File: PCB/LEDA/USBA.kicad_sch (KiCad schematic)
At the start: 22 parts, among them J1 USB_A, J2 Conn_01x03, T1 T3902_MEMS_Mic, U2 ESP32-S3-MINI-1, U5 MD8942

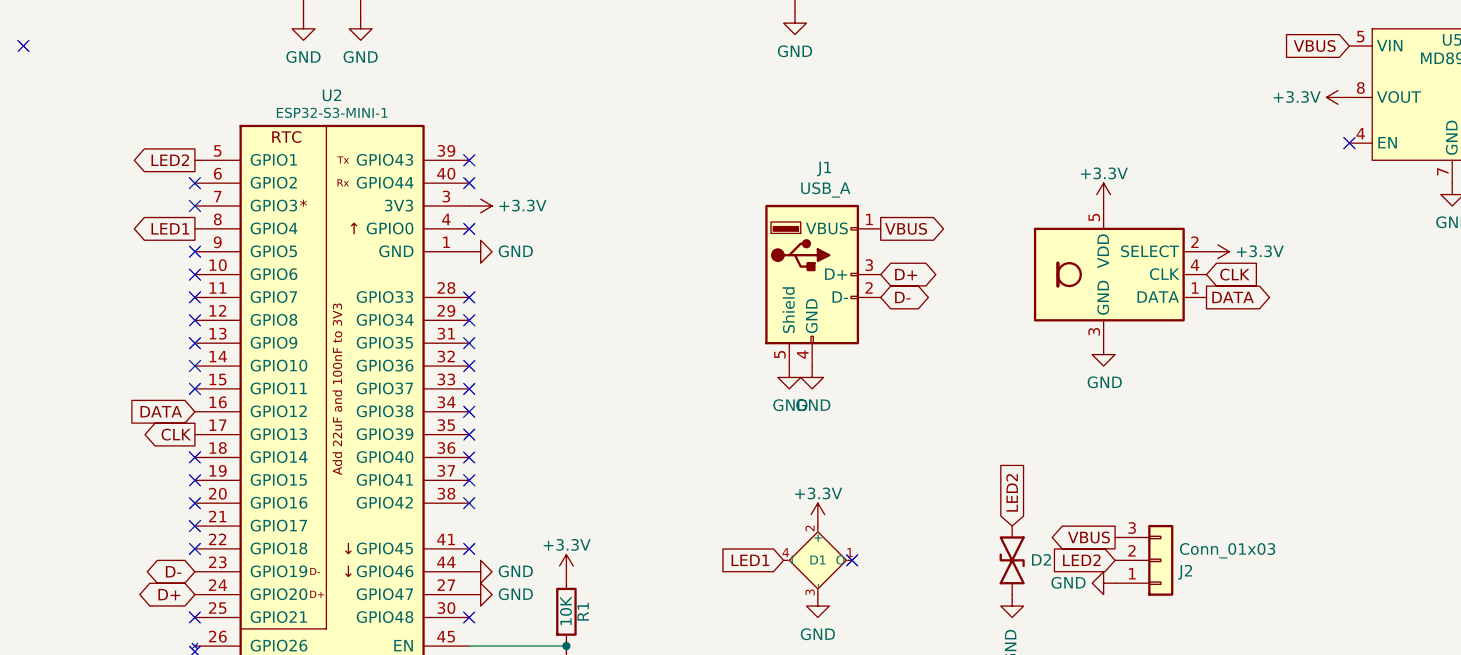
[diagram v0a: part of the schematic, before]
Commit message: New mic
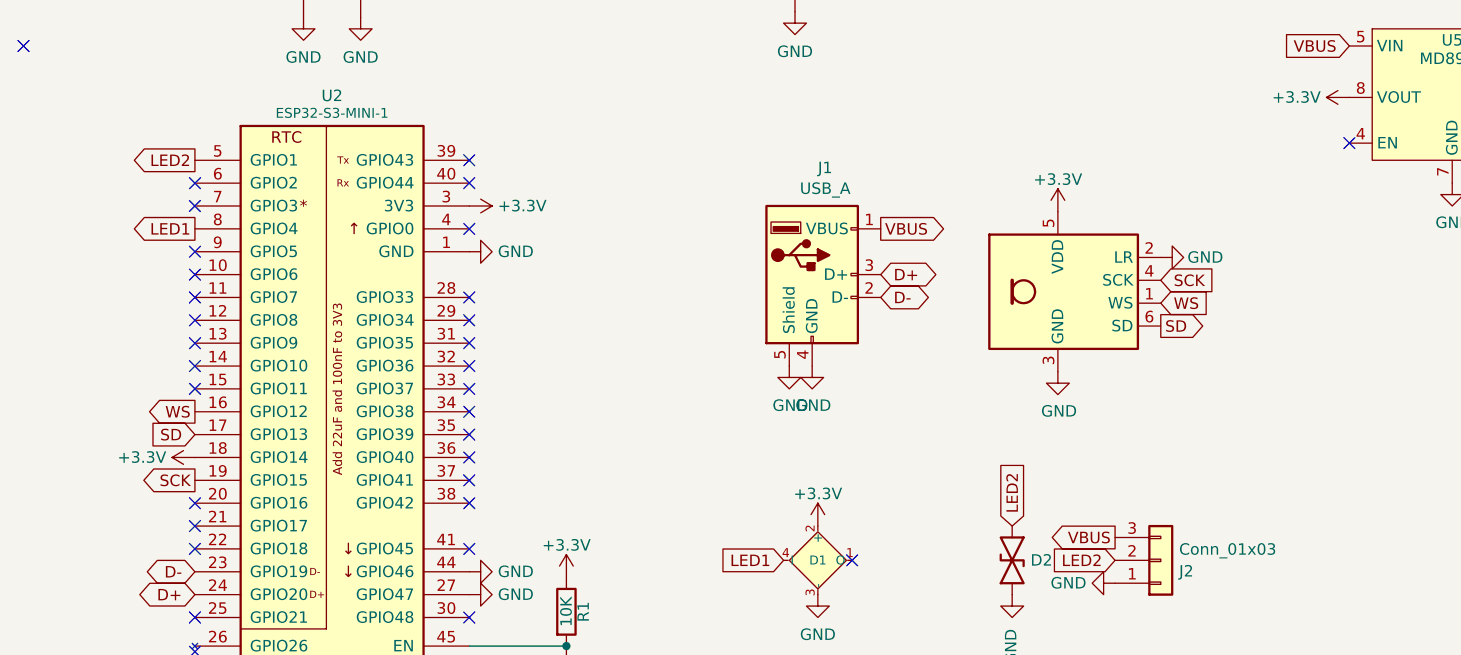
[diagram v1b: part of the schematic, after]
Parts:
- removed T1: T3902_MEMS_Mic, RevK:T3902_MEMS_Mic, symbol RevK:T3902_MEMS_Mic
- added U1: ICS43434_MEMS_Mic, RevK:ICS43434_MEMS_Mic, symbol RevK:ICS43434_MEMS_Mic
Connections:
- net +3.3V: now also U2.18 (GPIO14), U1.5 (VDD)
- net GND: now also U1.2 (LR), U1.3 (GND)
- net SCK: now reaches U2.19 (GPIO15)
- net SCK: now also U1.4 (SCK)
- net CLK renamed SD
- net SD: now also U1.6 (SD)
- net DATA renamed WS
- net WS: now also U1.1 (WS)
- no-connect marks 34 -> 32
